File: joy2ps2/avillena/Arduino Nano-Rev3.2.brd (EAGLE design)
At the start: 128.4 x 49.3 mm, 30 parts, among them IC2 LM1117IMPX-5.0, IC3 ATMEGA328P-AU, SW1 RESET, Y1 16MHz

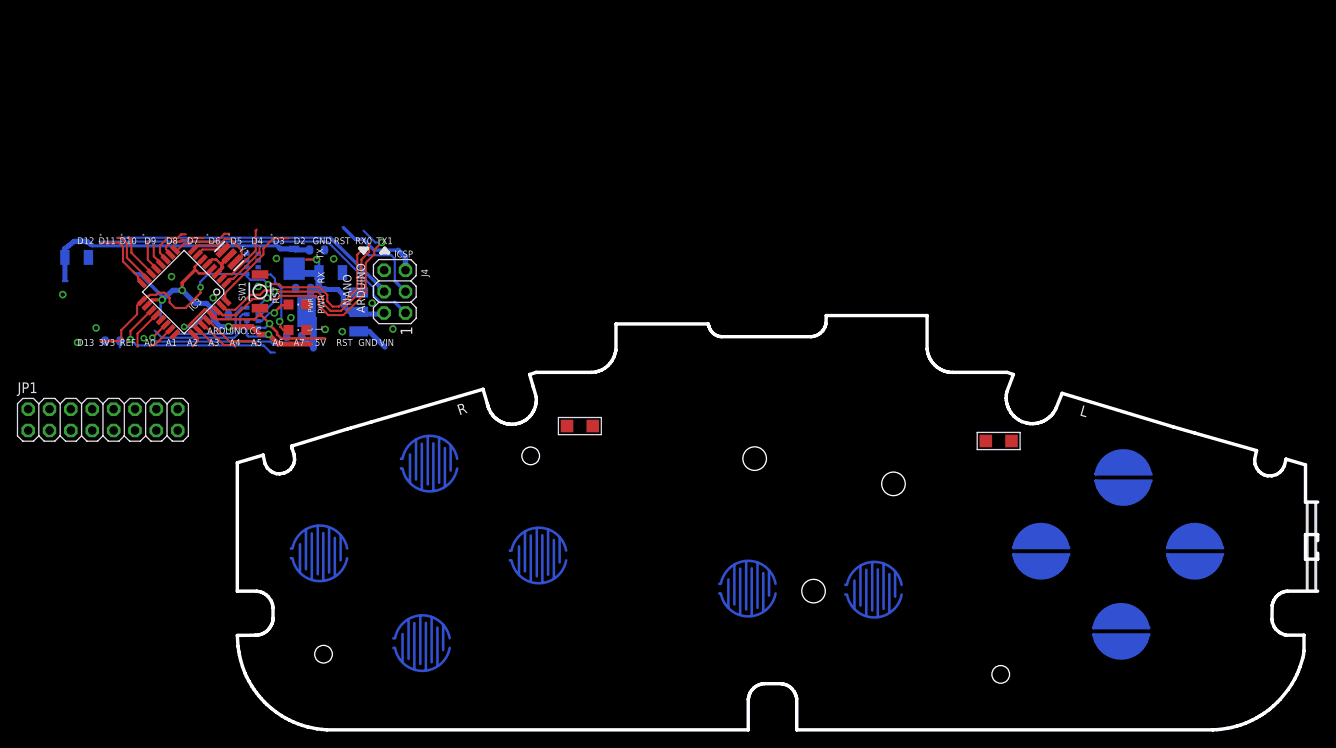
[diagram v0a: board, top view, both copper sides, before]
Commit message: A falta de vías
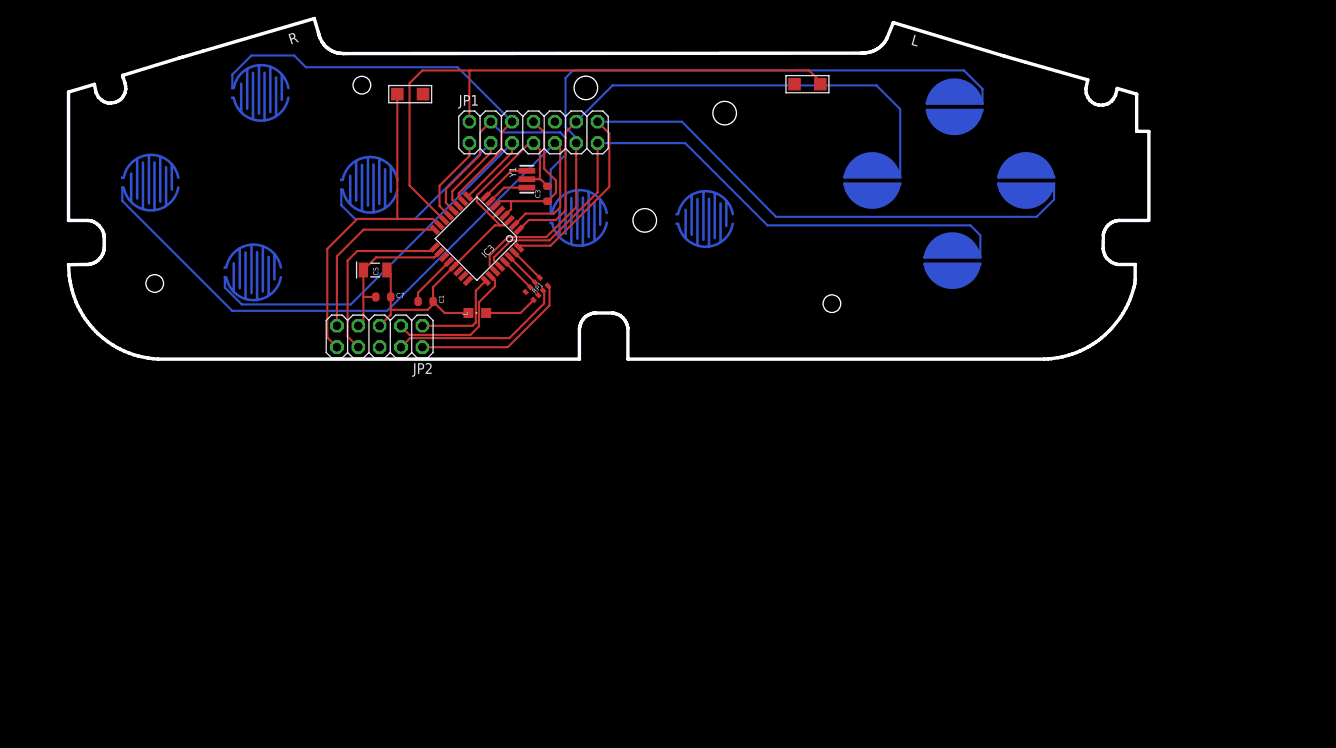
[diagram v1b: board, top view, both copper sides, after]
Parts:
- removed C2: 4,7uF_16V, Condensatori:TAN-A
- removed C8: 1uF, Condensatori:C0603-ROUND
- removed C9: 100nF, Condensatori:C0603-ROUND
- removed D1: SS1P3L, Diodi:DO220AAL
- removed IC2: LM1117IMPX-5.0, IntegratedCircuits:LINEAR_SOT223
- removed J4: (no value), Connettori:2X03
- removed PWR: Green, Opto:CHIPLED_0805
- removed RP2: 1K, Resistenze:CAY16
- removed SW1: RESET, Switches:SMD_157SW
- added JP2: (no value), pinhead:2X05
- JP1: device pinhead:2X08 -> pinhead:2X07
- moved JP1 61.5 mm to (57.0, 27.8)
- moved BTN-3 48.4 mm to (24.6, 32.5)
- moved BTN-4 48.4 mm to (115.6, 22.1)
- moved BTN-5 48.4 mm to (97.3, 22.1)
- moved BTN-6 48.4 mm to (11.6, 21.8)
- moved BTN-7 48.4 mm to (37.6, 21.6)
- moved BTN-8 48.4 mm to (106.8, 12.6)
- moved BTN-9 48.4 mm to (23.7, 11.2)
- moved BTN-DEL 48.4 mm to (77.5, 17.5)
- moved BTN-ENTER 48.4 mm to (62.5, 17.7)
- moved BTN-2 48.4 mm to (107.1, 30.9)
- moved BTN-0 48.1 mm to (89.5, 33.5)
- moved BTN-1 44.3 mm to (42.4, 32.4), turned to 180 degrees
- moved C3 41.4 mm to (58.7, 20.5), flipped to the top, turned to 90 degrees
- moved C1 37.5 mm to (44.2, 7.72), flipped to the top
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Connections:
- removed net COM: C1.2, C2.2, C3.2, C5.2, C7.2, C8.2, C9.2, IC2.1, IC3.21, IC3.3, IC3.5, J4.6, JP1.1, L.C, PWR.C, RP2.3, RP2.6, SW1.1, Y1.2
- removed net N$3: PWR.A, RP1.3
- removed net VIN: IC2.3
- removed net VUSB: C2.1, C9.1, D1.P$2
- net +5V: now also JP2.7; no longer C8.1, D1.P$1, IC2.2, IC2.4, J4.2, RP1.5
- net A2: now also JP2.1
- net A3: now also JP2.3; no longer JP1.9
- net A4: now also JP1.11; no longer JP1.15
- net A5: now also JP1.13; no longer JP1.7
- net D0/RX: now also RP1.2; no longer RP1.1
- net D1/TX: now also RP1.1; no longer RP1.2
- net D10: now also JP1.2; no longer JP1.10
- net D11/MOSI: now also JP1.10, JP2.10; no longer J4.4, JP1.2
- net D12/MISO: now also JP2.9; no longer J4.1
- net D13/SCK: now also JP2.8, RP1.4; no longer J4.3, RP2.1
- net D3: now also JP1.12; no longer JP1.6
- net D4: now also JP1.9; no longer JP1.13
- net D6: now also JP1.6; no longer JP1.12
- net D7: now also JP1.3; no longer JP1.4
- net D8: now also JP1.4; no longer JP1.11
- net D9: now also JP1.1; no longer JP1.3
- net GND: now also C1.2, C3.2, C5.2, C7.2, IC3.21, IC3.3, IC3.5, JP1.7, JP2.5, L.C, Y1.2
- net N$7: now also RP1.5; no longer RP2.8
- net RESET: now also JP2.6, RP1.3; no longer J4.5, RP1.4, SW1.2
- net RX: now also JP2.4, RP1.7; no longer RP1.8
- net TX: now also JP2.2, RP1.8; no longer RP1.7
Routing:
- net A4: track 5.63 -> 83.3 mm
- net D4: track 8.44 -> 80.9 mm
- net D2: track 11.7 -> 83.7 mm
- net D10: track 5.81 -> 74.5 mm
- net A5: track 7.49 -> 75.4 mm
- net D3: track 6.25 -> 67.1 mm
- net GND: track 0.00 -> 54.5 mm
- net D5: track 7.31 -> 52.7 mm
- net D6: track 6.35 -> 51.4 mm
- net +5V: track 74.4 -> 37.7 mm, vias 5 -> 0
- net VUSB: track 34.5 -> 0.00 mm
- net D13/SCK: track 54.7 -> 21.8 mm, vias 3 -> 0
- net RESET: track 36.3 -> 4.29 mm, vias 2 -> 0
- net D8: track 2.92 -> 32.5 mm
- net D0/RX: track 33.0 -> 4.29 mm, vias 2 -> 0
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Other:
- board size 128.4 x 49.3 mm -> 128.4 x 40.5 mm
- board text removed: "*"
- board text removed: "1"
- board text removed: "3V3"
- board text removed: "5V"
- board text removed: "A0"
- board text removed: "A1"
- board text removed: "A2"
- board text removed: "A3"
- board text removed: "A4"
- board text removed: "A5"
- board text removed: "A6"
- board text removed: "A7"
- board text removed: "ARDUINO"
- board text removed: "ARDUINO.CC"
- board text removed: "D10"
- board text removed: "D11"
- board text removed: "D12"
- board text removed: "D13"
- board text removed: "D2"
- board text removed: "D3"
- board text removed: "D4"
- board text removed: "D5"
- board text removed: "D6"
- board text removed: "D7"
- board text removed: "D8"
- board text removed: "D9"
- board text removed: "GND"
- board text removed: "ICSP"
- board text removed: "NANO"
- board text removed: "PWR"
- board text removed: "REF"
- board text removed: "RST"
- board text removed: "RX"
- board text removed: "RX0"
- board text removed: "TX"
- board text removed: "TX1"
- board text removed: "VIN"
